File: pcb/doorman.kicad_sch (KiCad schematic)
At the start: 41 parts, among them J1 USB_C_Receptacle_USB2.0, J2 Terminal, J3 3V3 Test Pad, J4 TX Test Pad, J5 RX Test Pad, J6 BUS Test Pad, J7 BUS RX Test Pad, Q1 BC817, SW1 Reset Button, SW2 Flash Button, U1 ESP32-S3-WROOM-1, U2 AP63203WU, U3 GAQY252G3S

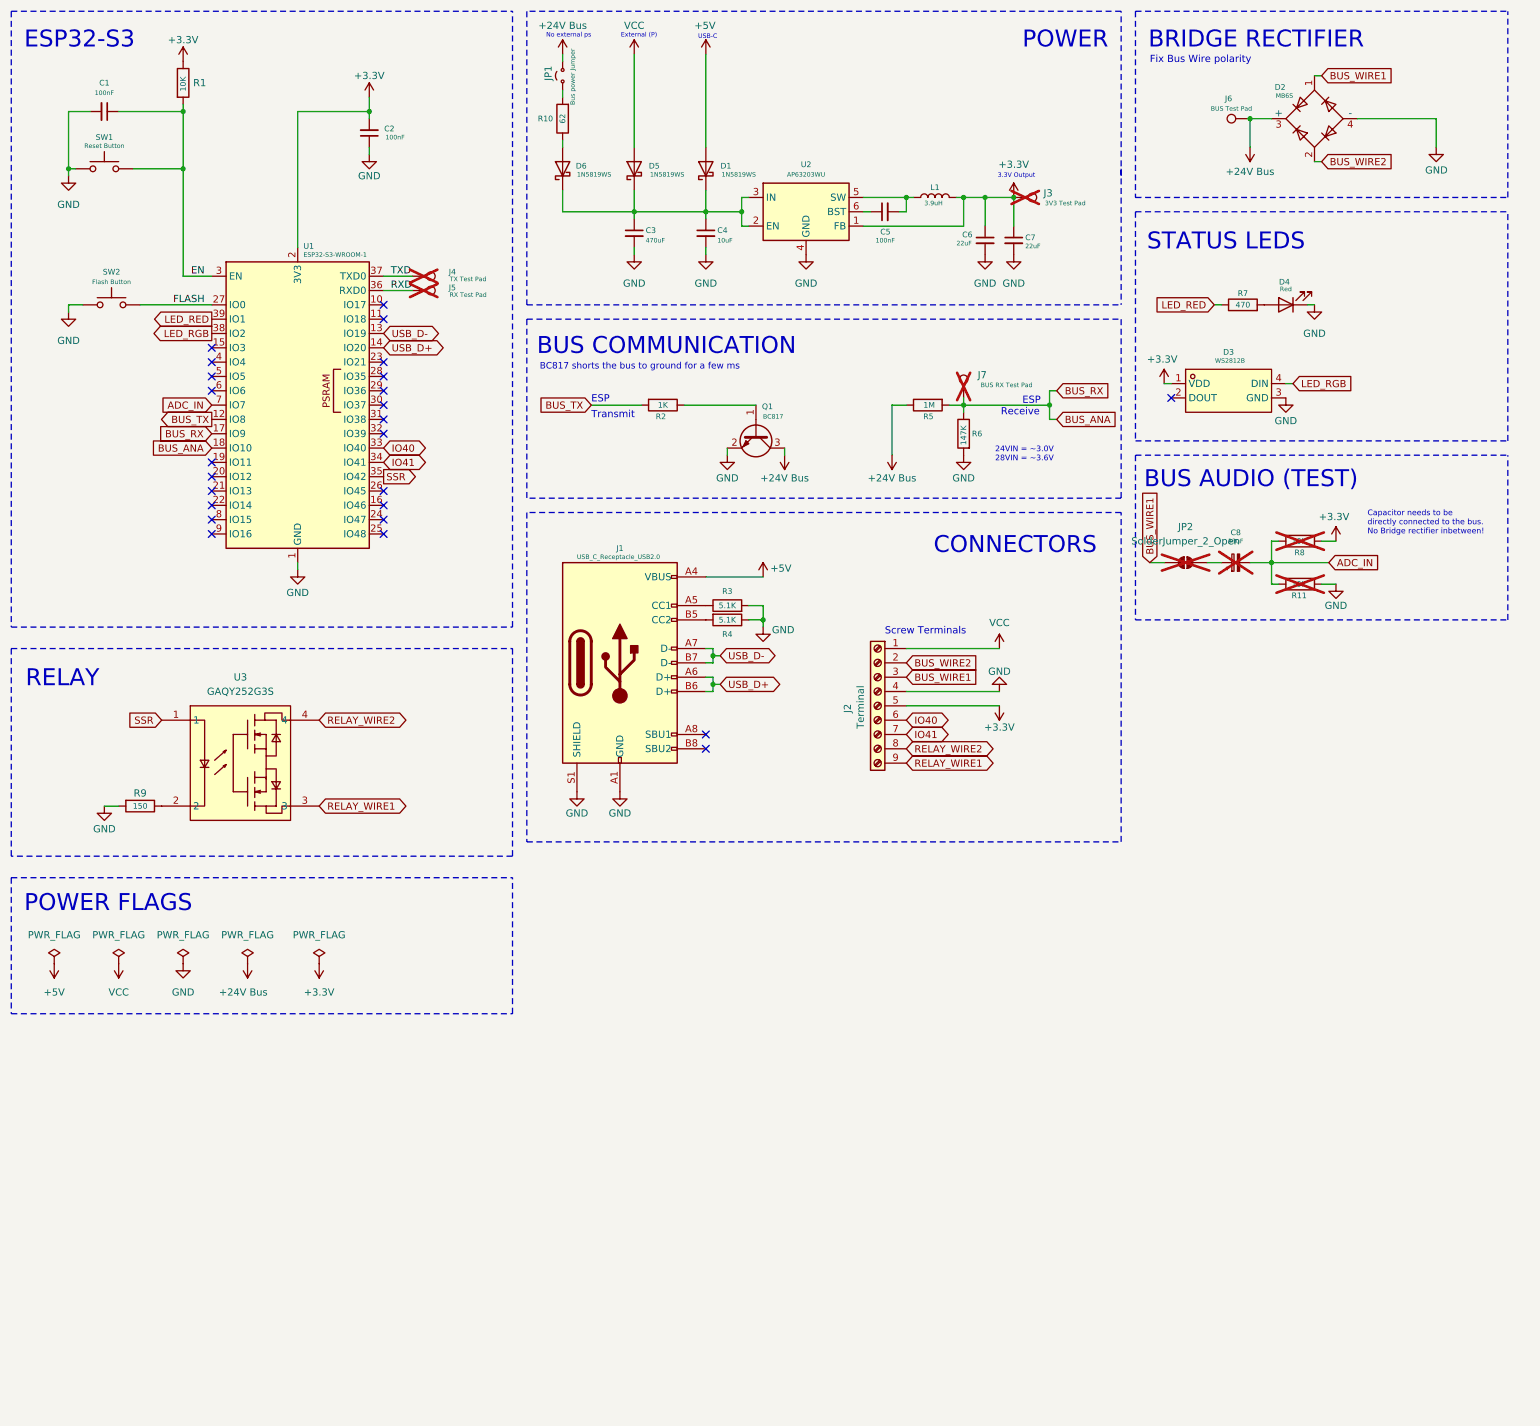
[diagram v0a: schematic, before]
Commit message: WIP
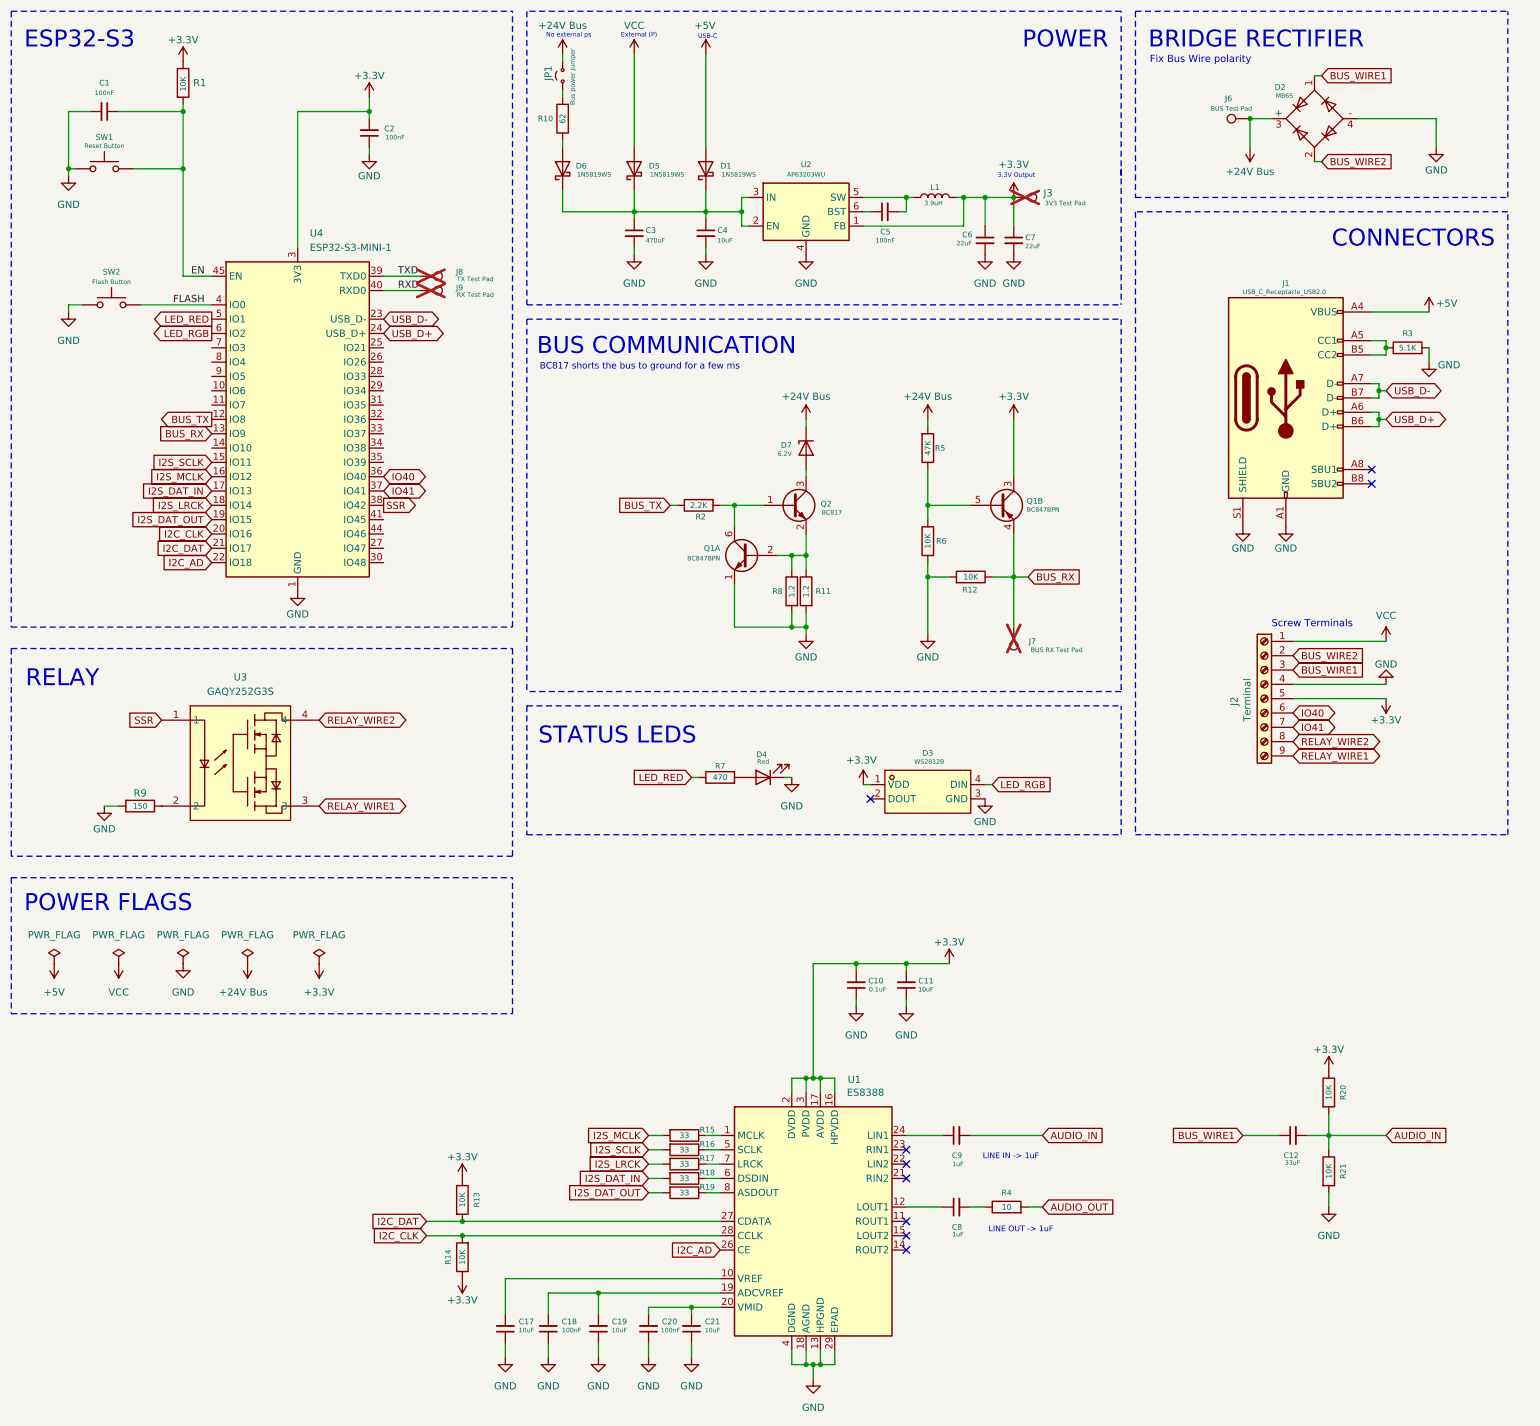
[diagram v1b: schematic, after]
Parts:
- removed C8: 33uF, Capacitor_SMD:C_1206_3216Metric_Pad1.33x1.80mm_HandSolder, symbol Device:C_Polarized_Small
- removed J4: TX Test Pad, TestPoint:TestPoint_Pad_D1.0mm, symbol Connector:TestPoint
- removed J5: RX Test Pad, TestPoint:TestPoint_Pad_D1.0mm, symbol Connector:TestPoint
- removed JP2: SolderJumper_2_Open, Jumper:SolderJumper-2_P1.3mm_Open_RoundedPad1.0x1.5mm, symbol Jumper:SolderJumper_2_Open
- removed U1: ESP32-S3-WROOM-1, RF_Module:ESP32-S3-WROOM-1, symbol RF_Module:ESP32-S3-WROOM-1
- added C10: 0.1uF, Capacitor_SMD:C_0603_1608Metric, symbol Device:C_Small
- added C11, C17, C19, C21: 10uF, Capacitor_SMD:C_0603_1608Metric, symbol Device:C_Small
- added C12: 33uF, Capacitor_SMD:C_1206_3216Metric, symbol Device:C_Small
- added C18, C20: 100nF, Capacitor_SMD:C_0603_1608Metric, symbol Device:C_Small
- added C8, C9: 1uF, Capacitor_SMD:C_0603_1608Metric, symbol Device:C_Small
- added D7: 6.2V, Diode_SMD:D_MELF, symbol Diode:BZV55C6V2
- added J8: TX Test Pad, TestPoint:TestPoint_Pad_D1.0mm, symbol Connector:TestPoint
- added J9: RX Test Pad, TestPoint:TestPoint_Pad_D1.0mm, symbol Connector:TestPoint
- added Q1: BC847BPN, Package_TO_SOT_SMD:SOT-363_SC-70-6, symbol Transistor_BJT:BC847BPN
- added R12, R20, R21: 10K, Resistor_SMD:R_0603_1608Metric, symbol Device:R
- added R13, R14: 10K, Resistor_SMD:R_0402_1005Metric, symbol Device:R
- added R15, R16, R17, R18, R19: 33, Resistor_SMD:R_0402_1005Metric, symbol Device:R
- added U1: ES8388, Package_DFN_QFN:QFN-28-1EP_4x4mm_P0.45mm_EP2.6x2.6mm, symbol Audio:ES8388
- added U4: ESP32-S3-MINI-1, RF_Module:ESP32-S2-MINI-1, symbol RF_Module:ESP32-S3-MINI-1
- Q2: renamed from Q1; LCSC C5184412 -> C609806; MPN BC817-25 -> BC817-40
- R11, R8: value 10K -> 1.2; footprint Resistor_SMD:R_1206_3216Metric_Pad1.30x1.75mm_HandSolder -> Resistor_SMD:R_0805_2012Metric; LCSC C25804 -> C2933356; MPN 0603WAF1002T5E -> FRC0805F1R20TS; Package 0603 -> 0805; now fitted; now in the parts list
- R2: value 1K -> 2.2K; LCSC C11702 -> C25879; MPN 0402WGF1001TCE -> 0402WGF2201TCE
- R4: value 5.1K -> 10
- R5: value 1M -> 47K
- R6: value 147K -> 10K
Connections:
- net ADC_IN is gone; now on net GND: R11.2, R8.2
- net +24V Bus: now also R5.2, D7.1 (K); no longer Q2.3 (C), R5.1
- net +3.3V: now also C10.2, C11.2, Q1.3 (C2), R13.1, R14.1, R20.1, U1.16 (HPVDD), U1.17 (AVDD), U1.2 (DVDD), U1.3 (PVDD), U4.3 (3V3); no longer R8.1
- net BUS_TX: now also R2.1, U4.12 (IO8); no longer R2.2
- net BUS_WIRE1: now also C12.1
- net EN: now also U4.45 (EN)
- net FLASH: now also U4.4 (IO0)
- net GND: now also C10.1, C11.1, C17.1, C18.1, C19.1, C20.1, C21.1, Q1.1 (E1), R12.2, R21.2, U1.13 (HPGND), U1.18 (AGND), U1.29 (EPAD), U1.4 (DGND), U4.1 (GND), U4.2 (GND), U4.42 (GND), U4.43 (GND), U4.46 (GND), U4.47 (GND), U4.48 (GND), U4.49 (GND), U4.50 (GND), U4.51 (GND), U4.52 (GND), U4.53 (GND), U4.54 (GND), U4.55 (GND), U4.56 (GND), U4.57 (GND), U4.58 (GND), U4.59 (GND), U4.60 (GND), U4.61 (GND), U4.62 (GND), U4.63 (GND), U4.64 (GND), U4.65 (GND); no longer Q2.2 (E), R11.1, R4.1
- net IO40: now also U4.36 (IO40)
- net IO41: now also U4.37 (IO41)
- net LED_RED: now also U4.5 (IO1)
- net LED_RGB: now also U4.6 (IO2)
- net RXD: now also J9.1, U4.40 (RXD0)
- net SSR: now also U4.38 (IO42)
- net TXD: now also J8.1, U4.39 (TXD0)
- net USB_D+: now also U4.24 (USB_D+)
- net USB_D-: now also U4.23 (USB_D-)
- net at J1.A5 (CC1), R3.1: now also J1.B5 (CC2)
- net AUDIO_OUT: now reaches R4.2
- net AUDIO_OUT: no longer J1.B5 (CC2)
- net at Q2.1 (B): now also R2.2, Q1.6 (C1); no longer R2.1
- removed net BUS_ANA: J7.1, R5.2, R6.1
- new net: Q1.5 (B2), R5.1, R6.1
- new net: Q1.2 (B1), Q2.2 (E), R11.1, R8.1
- new net: D7.2 (A), Q2.3 (C)
- new net: R18.1, U1.6 (DSDIN)
- new net: R17.1, U1.7 (LRCK)
- new net: C17.2, U1.10 (VREF)
- new net: R16.1, U1.5 (SCLK)
- new net: C20.2, C21.2, U1.20 (VMID)
- new net: C18.2, C19.2, U1.19 (ADCVREF)
- new net: C8.2, R4.1
- new net: C8.1, U1.12 (LOUT1)
- new net: R15.1, U1.1 (MCLK)
- new net: C9.1, U1.24 (LIN1)
- new net: R19.1, U1.8 (ASDOUT)
- new net AUDIO_IN: C12.2, C9.2, R20.2, R21.1
- new net BUS_RX: J7.1, Q1.4 (E2), R12.1, U4.13 (IO9)
- new net I2C_AD: U1.26 (CE), U4.22 (IO18)
- new net I2C_CLK: R14.2, U1.28 (CCLK), U4.20 (IO16)
- new net I2C_DAT: R13.2, U1.27 (CDATA), U4.21 (IO17)
- new net I2S_DAT_IN: R18.2, U4.17 (IO13)
- new net I2S_DAT_OUT: R19.2, U4.19 (IO15)
- new net I2S_LRCK: R17.2, U4.18 (IO14)
- new net I2S_MCLK: R15.2, U4.16 (IO12)
- new net I2S_SCLK: R16.2, U4.15 (IO11)
- no-connect marks 25 -> 9
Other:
- note added: "LINE IN -> 1uF"
- note added: "LINE OUT -> 1uF"
- note removed: "24VIN = ~3.0V 28VIN = ~3.6V"
- note removed: "BUS AUDIO (TEST)"
- note removed: "Capacitor needs to be directly connected to the bus. No Bridge rectifier inbetween!"
- note removed: "ESP"
- note removed: "Receive"
- note removed: "Transmit"
- moved on the sheet: D3, D4, J1, J2, J7, Q2, R3, R6, R7
